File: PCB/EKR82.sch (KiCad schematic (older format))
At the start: 97 parts, among them J1 LED, J2 4PIN, P1 i2c_pin, P2 i2c_pin, SW1 SW_PUSH, SW10 SW_PUSH, SW11 SW_PUSH, SW12 SW_PUSH, SW13 SW_PUSH, SW14 SW_PUSH, SW15 SW_PUSH, SW16 SW_PUSH, SW17 SW_PUSH, SW18 SW_PUSH, SW19 SW_PUSH, SW2 SW_PUSH, SW20 SW_PUSH, SW21 SW_PUSH, SW22 SW_PUSH, SW23 SW_PUSH, SW24 SW_PUSH, SW25 SW_PUSH, SW26 SW_PUSH, SW27 SW_PUSH, SW28 SW_PUSH, SW29 SW_PUSH, SW3 SW_PUSH, SW30 SW_PUSH, SW31 SW_PUSH, SW32 SW_PUSH, SW33 SW_PUSH, SW34 SW_PUSH, SW35 SW_PUSH, SW36 SW_PUSH, SW37 SW_PUSH, SW38 SW_PUSH, SW39 SW_PUSH, SW4 SW_PUSH, SW40 SW_PUSH, SW41 SW_PUSH, SW5 SW_PUSH, SW6 SW_PUSH, SW7 SW_PUSH, SW8 SW_PUSH, SW9 SW_PUSH, U1 ProMicro

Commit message: rename kicad project EKR82_Pro to EKR82
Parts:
- D1, D10, D11, D12, D13, D14, D15, D16, D17, D18, D19, D2, D20, D21, D22, D23, D24, D25, D26, D27, D28, D29, D3, D30, D31, D32, D33, D34, D35, D36, D37, D38, D39, D4, D40, D41, D5, D6, D7, D8, D9: symbol EKR82_Pro-rescue:D-EKR82-cache -> EKR82-rescue:D-EKR82-cache
- J1: symbol EKR82_Pro-rescue:LED-EKR82-cache -> EKR82-rescue:LED-EKR82-cache
- J2: symbol EKR82_Pro-rescue:MJ-4PP-9-EKR82-cache -> EKR82-rescue:MJ-4PP-9-EKR82-cache
- P1, P2: symbol EKR82_Pro-rescue:i2c_pin-EKR82-cache -> EKR82-rescue:i2c_pin-EKR82-cache
- R1, R2: symbol EKR82_Pro-rescue:R-EKR82-cache -> EKR82-rescue:R-EKR82-cache
- RSW1: symbol EKR82_Pro-rescue:SW_RST-EKR82-cache -> EKR82-rescue:SW_RST-EKR82-cache
- SW1, SW10, SW11, SW12, SW13, SW14, SW15, SW16, SW17, SW18, SW19, SW2, SW20, SW21, SW22, SW23, SW24, SW25, SW26, SW27, SW28, SW29, SW3, SW30, SW31, SW32, SW33, SW34, SW35, SW36, SW37, SW38, SW39, SW4, SW40, SW41, SW5, SW6, SW7, SW8, SW9: symbol EKR82_Pro-rescue:SW_PUSH-EKR82-cache -> EKR82-rescue:SW_PUSH-EKR82-cache
- TH3, TH4, TH5, TH6, TH7, TH8: symbol EKR82_Pro-rescue:HOLE-EKR82-cache -> EKR82-rescue:HOLE-EKR82-cache
- U1: symbol EKR82_Pro-rescue:ProMicro_2-EKR82-cache -> EKR82-rescue:ProMicro_2-EKR82-cache

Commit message: move SW41 and remove resistors
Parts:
- removed R1, R2: R, EKR82-footprint:RESISTOR_mini, symbol EKR82-rescue:R-EKR82-cache
- removed W1: jumper, EKR82-footprint:jumper_data, symbol Device:Jumper

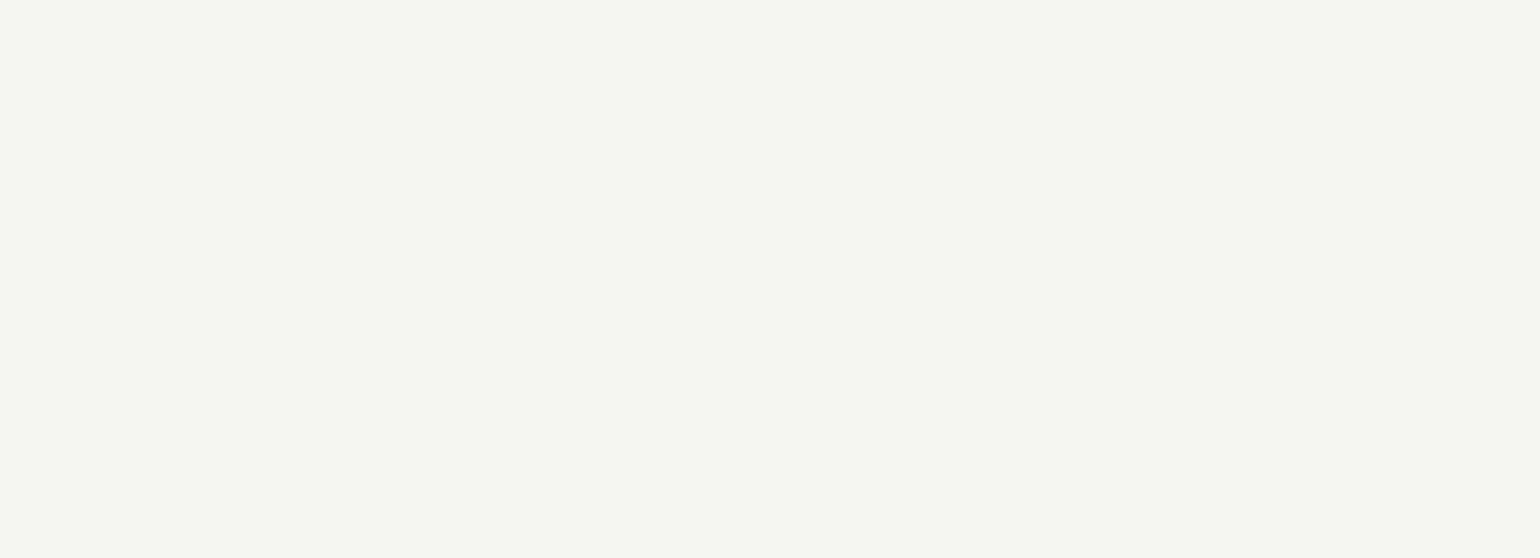
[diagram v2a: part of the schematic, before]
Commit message: add backlight rgb WIP
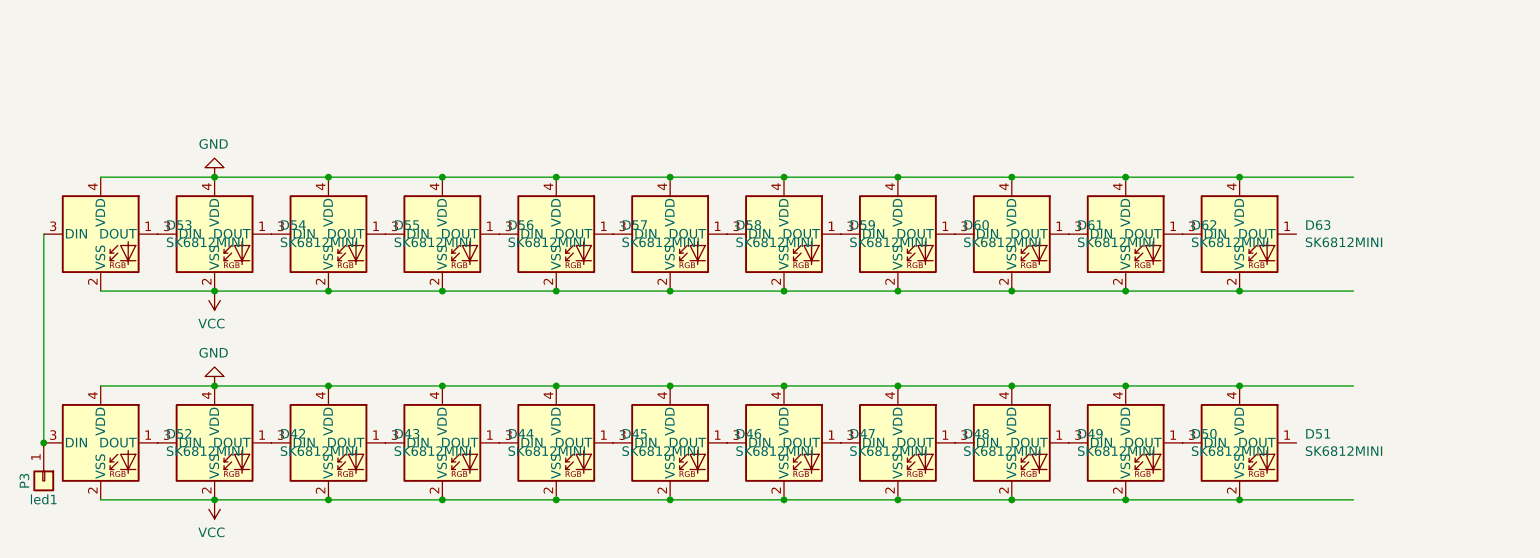
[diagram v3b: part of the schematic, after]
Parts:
- added D42, D43, D44, D45, D46, D47, D48, D49, D50, D51, D52, D53, D54, D55, D56, D57, D58, D59, D60, D61, D62, D63: SK6812MINI, LED_SMD:LED_SK6812MINI_PLCC4_3.5x3.5mm_P1.75mm, symbol LED:SK6812MINI
- added P3: led1, Connector_PinHeader_1.27mm:PinHeader_1x01_P1.27mm_Vertical, symbol EKR82-rescue:i2c_pin-EKR82-cache
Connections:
- wire segments 85 -> 130
